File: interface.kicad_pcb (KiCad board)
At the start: 2 copper layers, 36.8 x 66 mm, 35 parts, among them U1 THERMAL, U2 SX1308

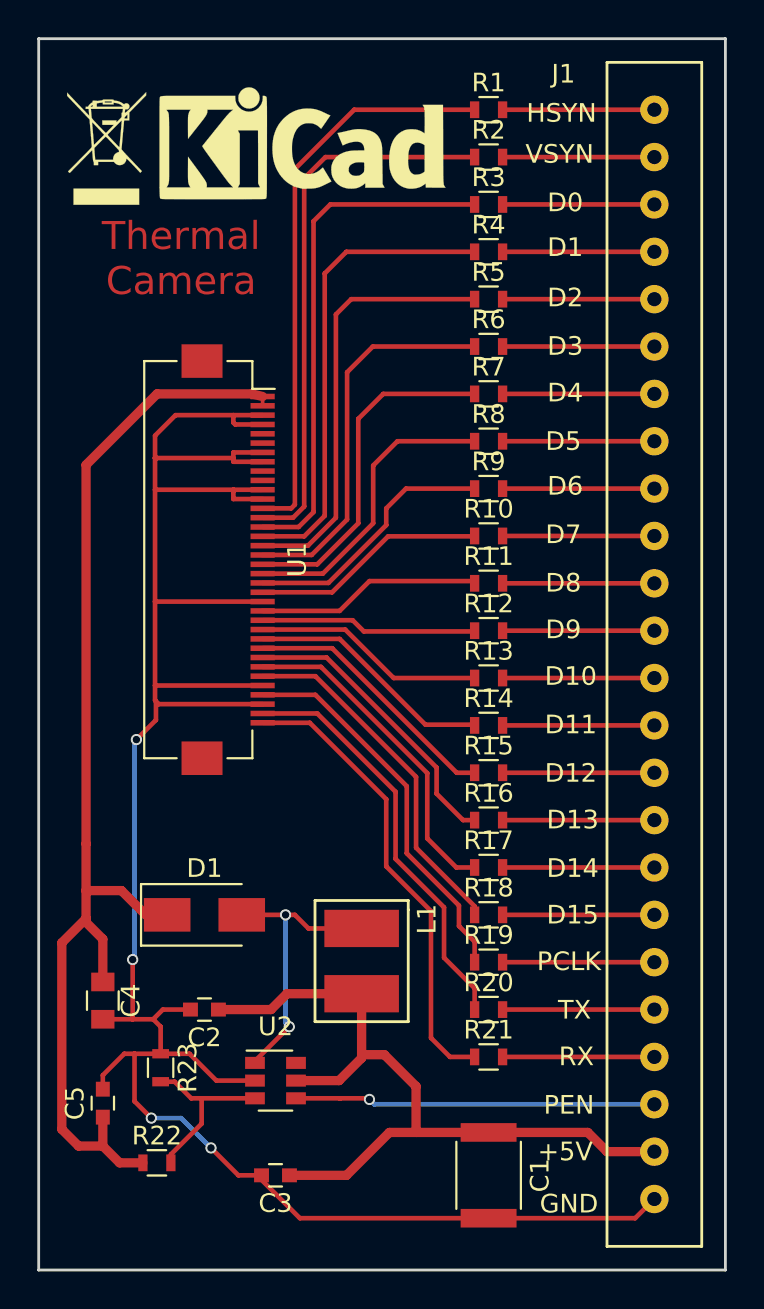
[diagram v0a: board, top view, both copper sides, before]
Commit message: finish pcb
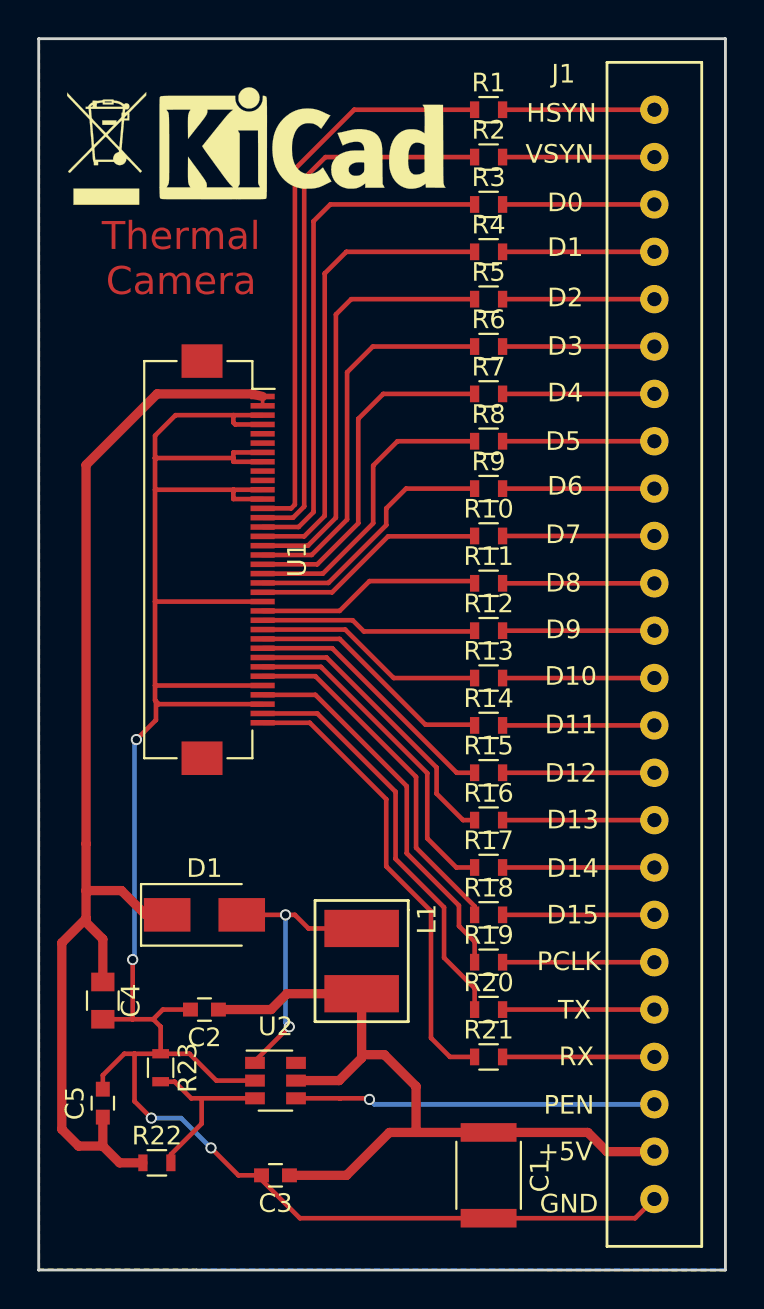
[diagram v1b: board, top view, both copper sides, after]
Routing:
- added copper zone on B.Cu, net GND
- added copper zone on F.Cu, net GND
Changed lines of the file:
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@@
   (segment (start 141.6 80.6) (end 141.6 75) (width 0.25) (layer F.Cu) (net 52))
   (segment (start 139.4 82.8) (end 141.6 80.6) (width 0.25) (layer F.Cu) (net 52))
+  (zone (net 2) (net_name GND) (layer F.Cu) (hatch edge 0.508)
+    (connect_pads (clearance 0.508))
+    (min_thickness 0.254)
+    (fill yes (arc_segments 16) (thermal_gap 0.508) (thermal_bridge_width 0.508))
+    (polygon
+      (pts
+        (xy 161.3 120.7) (xy 124.5 120.6) (xy 124.5 54.6) (xy 161.3 54.6)
+      )
+    )
+  )
+  (zone (net 2) (net_name GND) (layer B.Cu) (hatch edge 0.508)
+    (connect_pads (clearance 0.508))
+    (min_thickness 0.254)
+    (fill yes (arc_segments 16) (thermal_gap 0.508) (thermal_bridge_width 0.508))
+    (polygon
+      (pts
+        (xy 161.3 120.6) (xy 124.5 120.6) (xy 124.5 54.6) (xy 161.3 54.6)
+      )
+    )
+  )
 )
